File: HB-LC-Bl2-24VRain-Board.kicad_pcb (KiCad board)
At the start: 2 copper layers, 130 x 82.5 mm, 49 parts, among them IC1 ArduinoProMini, J1 Motor_N, J2 Taster Markise1, J3 Taster Markise 2, J4 Regensensor, J5 230V, J6 Motor1, J7 Motor2, Q1 BC337, Q2 BC337, Q3 BC337, Q4 BC337, SW1 SW_Push, U1 AM1S-2403S, U3 CC1101-868MHz-Module

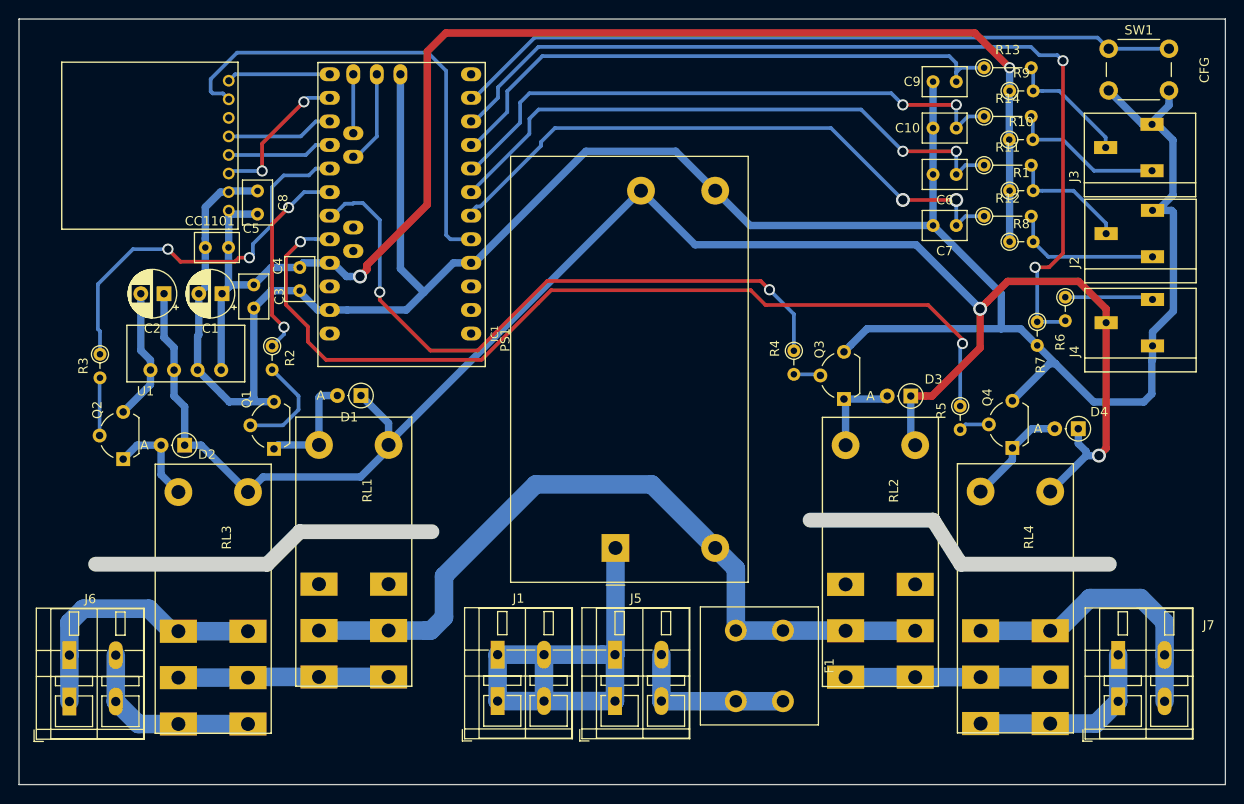
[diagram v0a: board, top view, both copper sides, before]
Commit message: Few updates to layout. But not yet done.
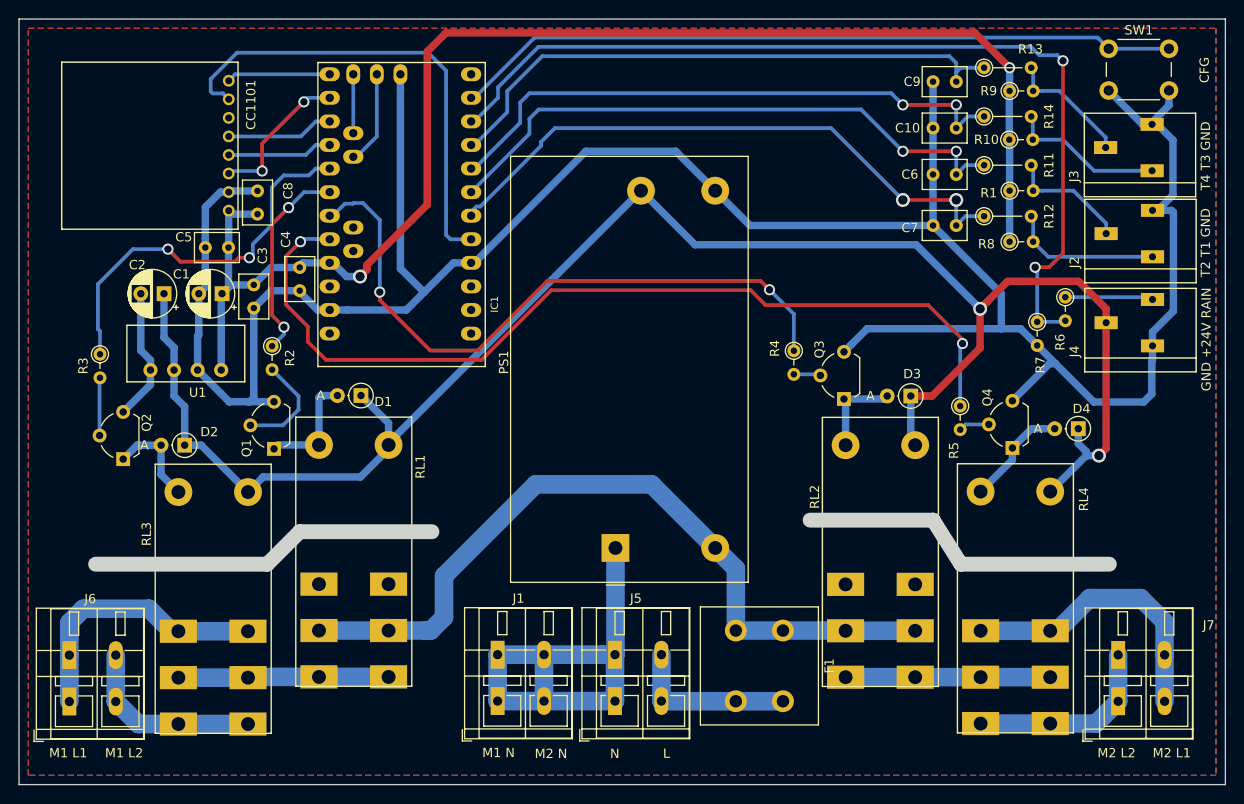
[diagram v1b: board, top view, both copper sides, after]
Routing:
- added copper zone on B.Cu, net GND
- added copper zone on F.Cu, net GND
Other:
- board text added: "M1 L2"
- board text removed: "M1_L2"
